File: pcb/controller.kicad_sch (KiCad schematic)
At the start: 58 parts, among them U2 SN65HVD230, U3 STM32F103RETx, Y2 8MHz, Y3 8MHz

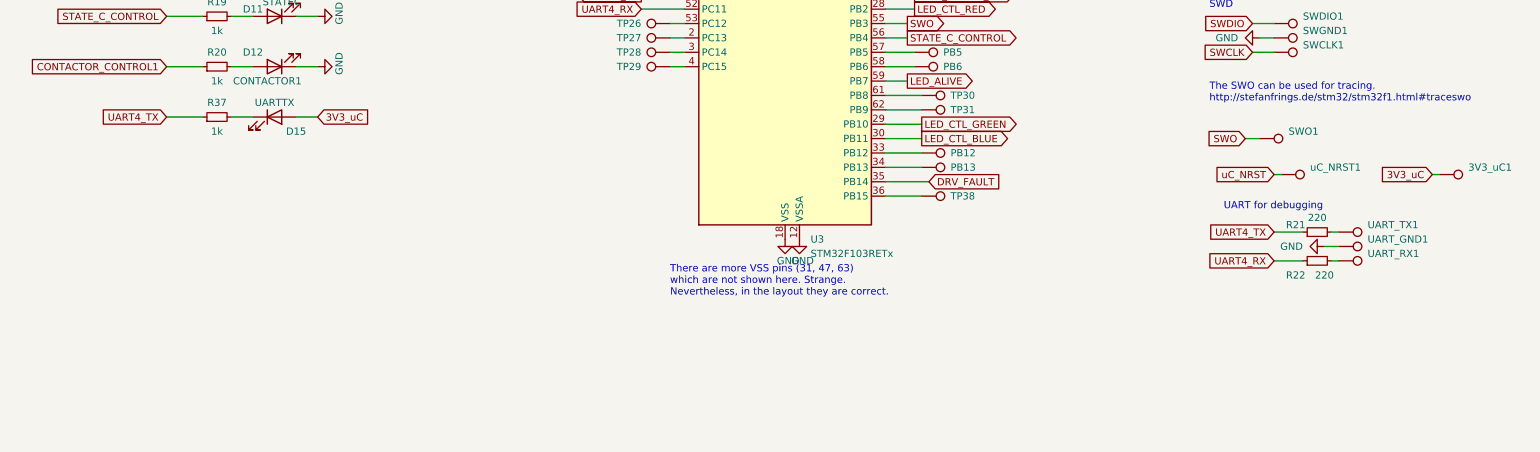
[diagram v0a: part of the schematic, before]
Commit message: added alternative 6-pin headers. Added uart3 test points. V5.2pre2
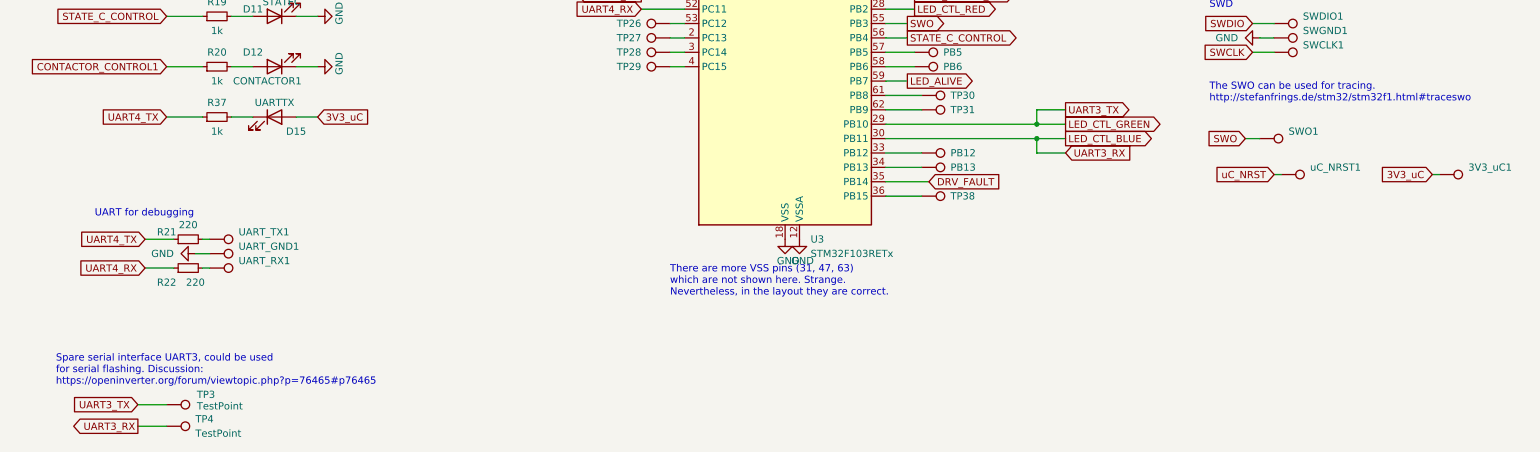
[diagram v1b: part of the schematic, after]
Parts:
- added TP3, TP4: TestPoint, speciallib:TestPoint_Special_THTPad_D1.9mm_Drill1mm, symbol Connector:TestPoint
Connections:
- net LED_CTL_BLUE: now also TP4.1
- net LED_CTL_GREEN: now also TP3.1
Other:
- note added: "Spare serial interface UART3, could be used for serial flashing. Discussion: https://openinverter.org/forum/viewtopic.php?p=76465#p76465"
- moved on the sheet: R21, R22, UART_GND1, UART_RX1, UART_TX1

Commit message: corrected some rotations for JLC. Version 5.2p7
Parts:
- U2, U3: JLCPCB Rotation Offset -90 -> 0
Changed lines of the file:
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@@
 			)
 		)
-		(property "JLCPCB Rotation Offset" "-90"
+		(property "JLCPCB Rotation Offset" "0"
 			(at 232.41 87.63 0)
 			(effects
@@
 			)
 		)
-		(property "JLCPCB Rotation Offset" "-90"
+		(property "JLCPCB Rotation Offset" "0"
 			(at 153.67 107.95 0)
 			(effects

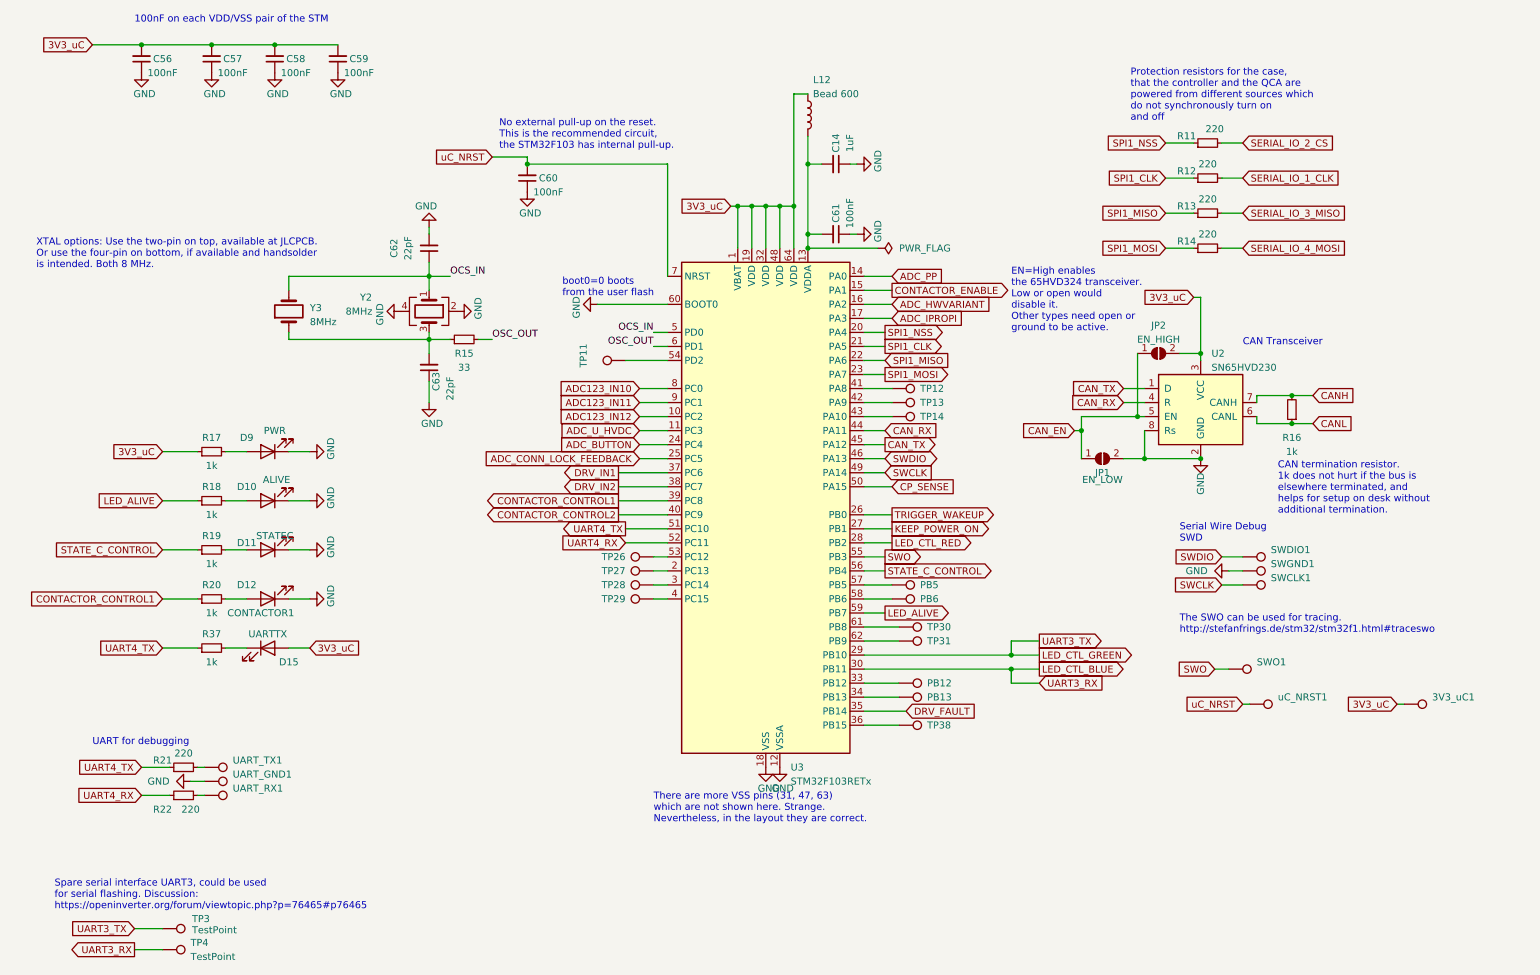
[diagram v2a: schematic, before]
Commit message: Added TC2030 for programming STM32
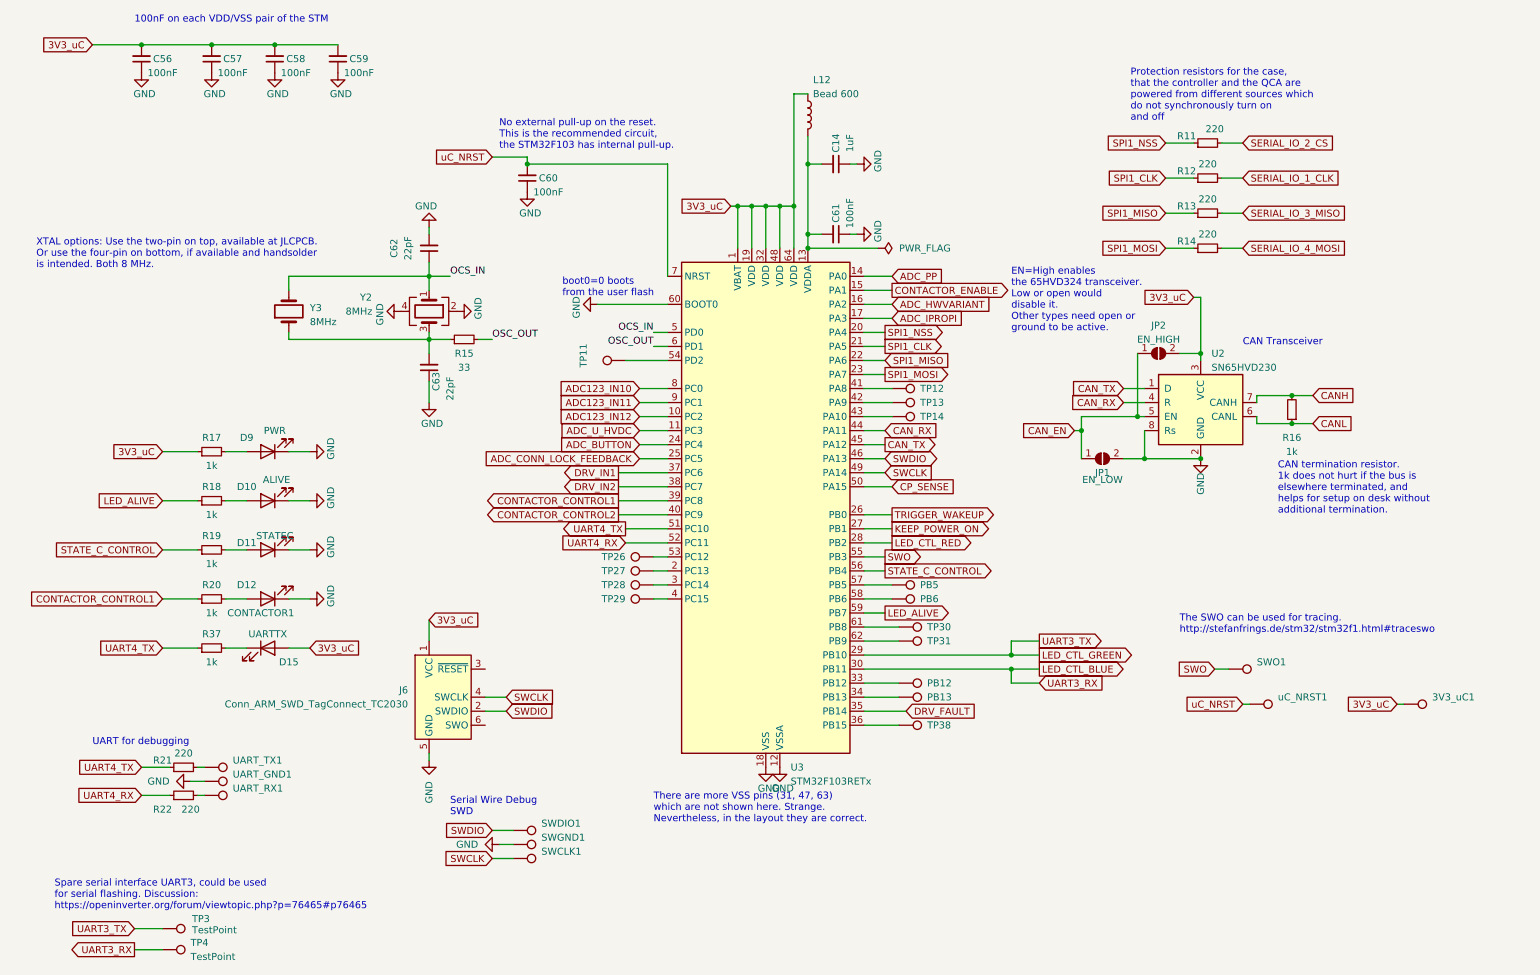
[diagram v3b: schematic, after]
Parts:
- added J6: Conn_ARM_SWD_TagConnect_TC2030, Connector:Tag-Connect_TC2030-IDC-FP_2x03_P1.27mm_Vertical, symbol Connector:Conn_ARM_SWD_TagConnect_TC2030
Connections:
- net 3V3_uC: now also J6.1 (VCC)
- net GND: now also J6.5 (GND)
- net SWCLK: now also J6.4 (SWCLK)
- net SWDIO: now also J6.2 (SWDIO)
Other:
- moved on the sheet: SWCLK1, SWDIO1, SWGND1
